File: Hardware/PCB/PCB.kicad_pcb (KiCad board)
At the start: 2 copper layers, 99.3 x 73.5 mm, 22 parts, among them J1 Conn_01x05_Pin, P1 USB_C_Plug, SW1 SW_HotSwap, U2 LP2985-3.3, U3 STM32F303RETx

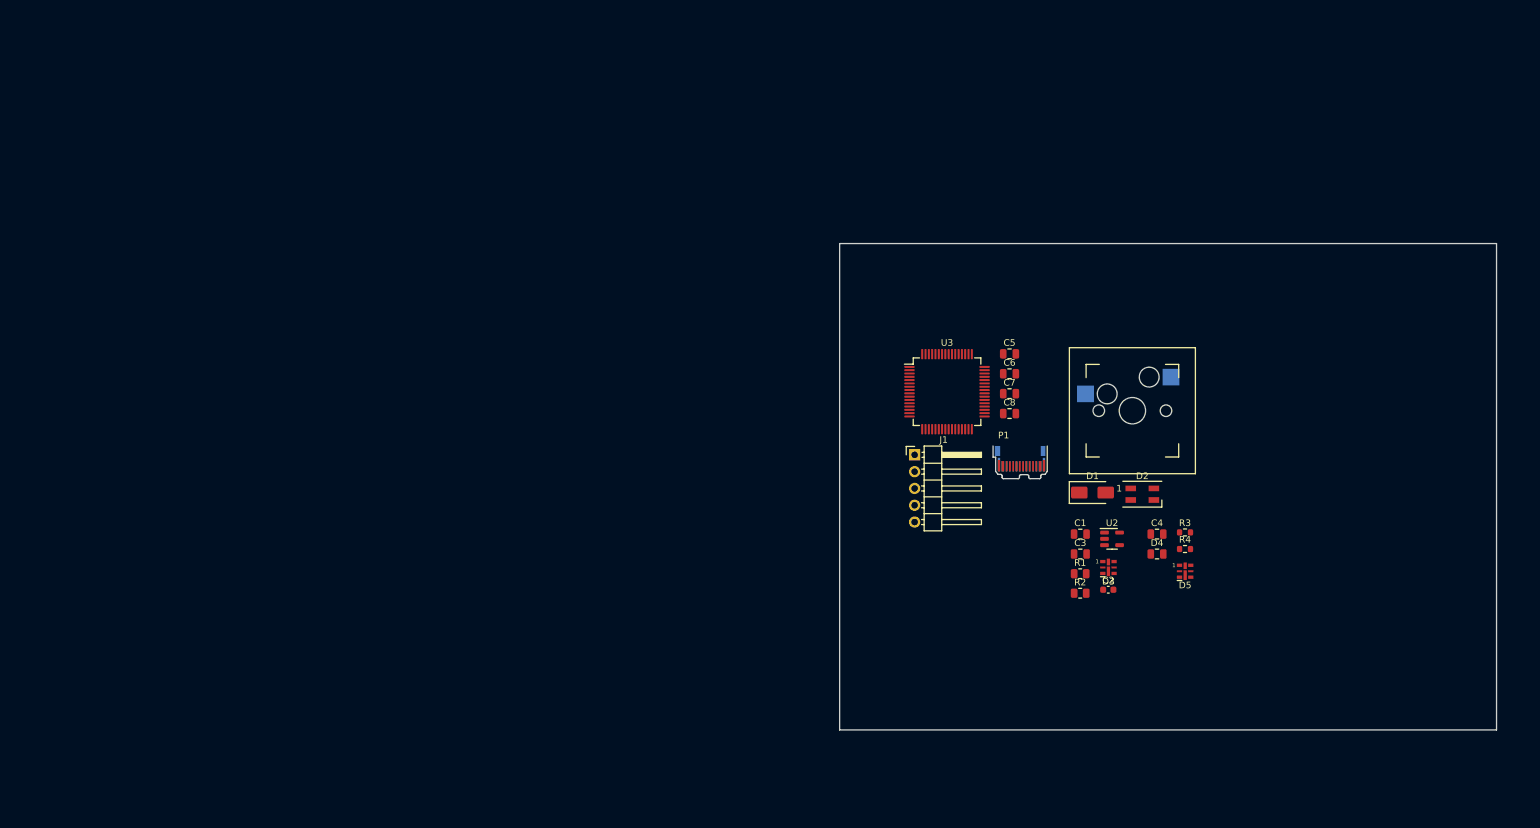
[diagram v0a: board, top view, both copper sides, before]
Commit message: Update of schematic and PCB
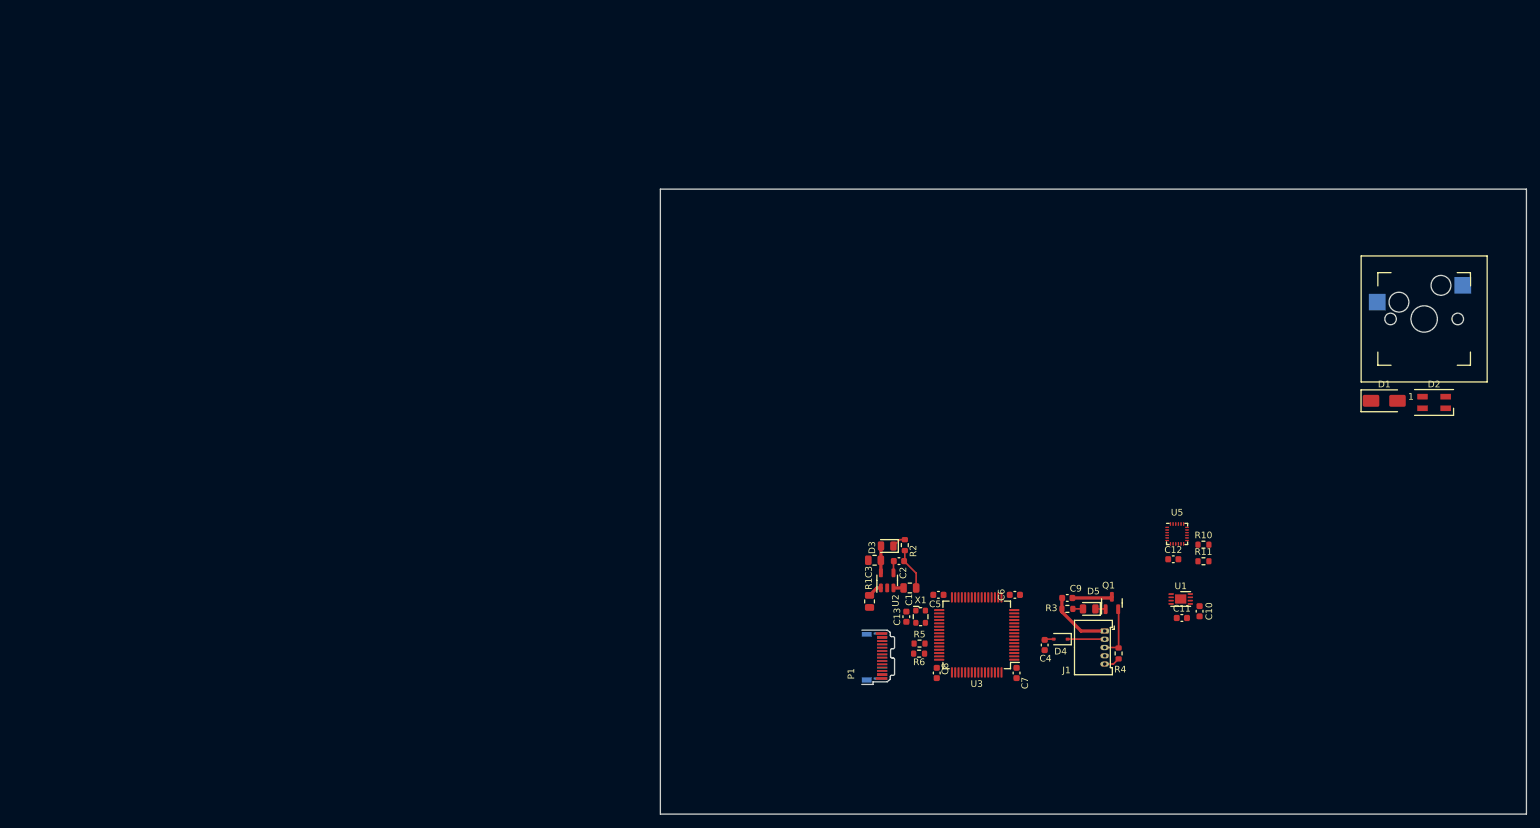
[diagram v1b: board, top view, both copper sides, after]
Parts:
- added C10: 100nF, Capacitor_SMD:C_0603_1608Metric, F.Cu at (199.0, 110.0)
- added C11: 100nF, Capacitor_SMD:C_0603_1608Metric, F.Cu at (196.3, 111.1)
- added C12: 100nF, Capacitor_SMD:C_0603_1608Metric, F.Cu at (195.0, 102.2)
- added C13: 100nF, Capacitor_SMD:C_0603_1608Metric, F.Cu at (154.7, 110.9)
- added C9: 100nF, Capacitor_SMD:C_0603_1608Metric, F.Cu at (179.0, 108.0)
- added Q1: NMOS, Package_TO_SOT_SMD:SOT-23, F.Cu at (185.7, 108.8)
- added R10: 4.7k, Resistor_SMD:R_0603_1608Metric, F.Cu at (199.6, 100.0)
- added R11: 4.7k, Resistor_SMD:R_0603_1608Metric, F.Cu at (199.6, 102.5)
- added R5: 0, Resistor_SMD:R_0603_1608Metric, F.Cu at (156.7, 114.9)
- added R6: 0, Resistor_SMD:R_0603_1608Metric, F.Cu at (156.6, 116.5)
- added U1: MCP98243, Package_DFN_QFN:DFN-8-1EP_3x2mm_P0.5mm_EP1.7x1.4mm, F.Cu at (196.1, 108.2)
- added U5: ICM-20948, Sensor_Motion:InvenSense_QFN-24_3x3mm_P0.4mm, F.Cu at (195.6, 98.4)
- added X1: ECS-2520MV-250-DN-TR, Oscillator:Oscillator_SMD_ECS_2520MV-xxx-xx-4Pin_2.5x2.0mm, F.Cu at (156.8, 110.9)
- C4, C5, C6, C7, C8: footprint Capacitor_SMD:C_0805_2012Metric -> Capacitor_SMD:C_0603_1608Metric
- D3, D5: footprint LED_SMD:LED-APA102-2020 -> LED_SMD:LED_0805_2012Metric
- D4: value 1N4818 -> BAS16HT1G; footprint Capacitor_SMD:C_0805_2012Metric -> Diode_SMD:D_SOD-323
- J1: value Conn_01x05_Pin -> 53048-0510; footprint Connector_PinHeader_2.54mm:PinHeader_1x05_P2.54mm_Horizontal -> Connector_Molex:Molex_PicoBlade_53048-0510_1x05_P1.25mm_Horizontal
- R2: footprint Resistor_SMD:R_0805_2012Metric -> Resistor_SMD:R_0603_1608Metric
- moved D1 46.2 mm to (226.9, 78.2)
- moved D2 46.2 mm to (234.4, 78.5)
- moved SW1 46.2 mm to (232.9, 65.9)
- moved C7 42.2 mm to (171.3, 119.4), turned to -90 degrees
- moved C8 40.7 mm to (159.3, 119.4), turned to 90 degrees
- moved J1 39.2 mm to (184.6, 113.0), turned to -90 degrees
- moved C5 38.0 mm to (159.5, 107.6), turned to 180 degrees
- moved P1 37.2 mm to (149.9, 116.8), turned to 90 degrees
- moved U3 37.0 mm to (165.3, 113.6), turned to 180 degrees
- moved U2 34.6 mm to (151.8, 105.4), turned to 90 degrees
- moved D3 33.6 mm to (151.8, 100.2), turned to 180 degrees
- moved C6 33.4 mm to (171.1, 107.6), turned to 180 degrees
- moved R1 32.1 mm to (149.1, 108.6), turned to 90 degrees
- moved C2 31.9 mm to (153.5, 102.5)
- moved C3 31.1 mm to (149.9, 102.3), turned to 180 degrees
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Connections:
- C4 pad 1: /Programming/NRST_OUT -> /MCU/NRST
- C5 pad 1: +3.3V -> /MCU/VCC_IN
- C6 pad 1: +3.3V -> /MCU/VCC_IN
- C7 pad 1: +3.3V -> /MCU/VCC_IN
- C8 pad 1: +3.3V -> /MCU/VCC_IN
- D4 pad 2: /Programming/NRST_OUT -> /MCU/NRST
- U3 pad 1: +3.3V -> /MCU/VCC_IN
- U3 pad 13: +3.3V -> /MCU/VCC_IN
- U3 pad 19: +3.3V -> /MCU/VCC_IN
- U3 pad 32: +3.3V -> /MCU/VCC_IN
- U3 pad 44: unconnected-(U3-PA11-Pad44) -> Net-(U3-PA11)
- U3 pad 45: unconnected-(U3-PA12-Pad45) -> Net-(U3-PA12)
- U3 pad 48: +3.3V -> /MCU/VCC_IN
- U3 pad 5: unconnected-(U3-PF0-Pad5) -> Net-(U3-PF0)
- U3 pad 64: +3.3V -> /MCU/VCC_IN
- U3 pad 7: unconnected-(U3-NRST-Pad7) -> /MCU/NRST
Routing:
- net GND: track 0.00 -> 14.9 mm
- net +5V: track 0.00 -> 9.77 mm
- net /Programming/SWD_IN: track 0.00 -> 8.02 mm
- net /Programming/NRST_IN: track 0.00 -> 5.61 mm
- net +3.3V: track 0.00 -> 4.08 mm
- net Net-(U2-ON/~{OFF}): track 0.00 -> 3.71 mm
- net Net-(D3-K): track 0.00 -> 2.12 mm
- net Net-(U2-BP): track 0.00 -> 1.81 mm
- net Net-(D5-K): track 0.00 -> 1.56 mm
- net Net-(D5-A): track 0.00 -> 1.54 mm
- net /MCU/NRST: track 0.00 -> 1.41 mm
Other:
- board size 99.3 x 73.5 mm -> 130.9 x 94.5 mm

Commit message: Update schematic
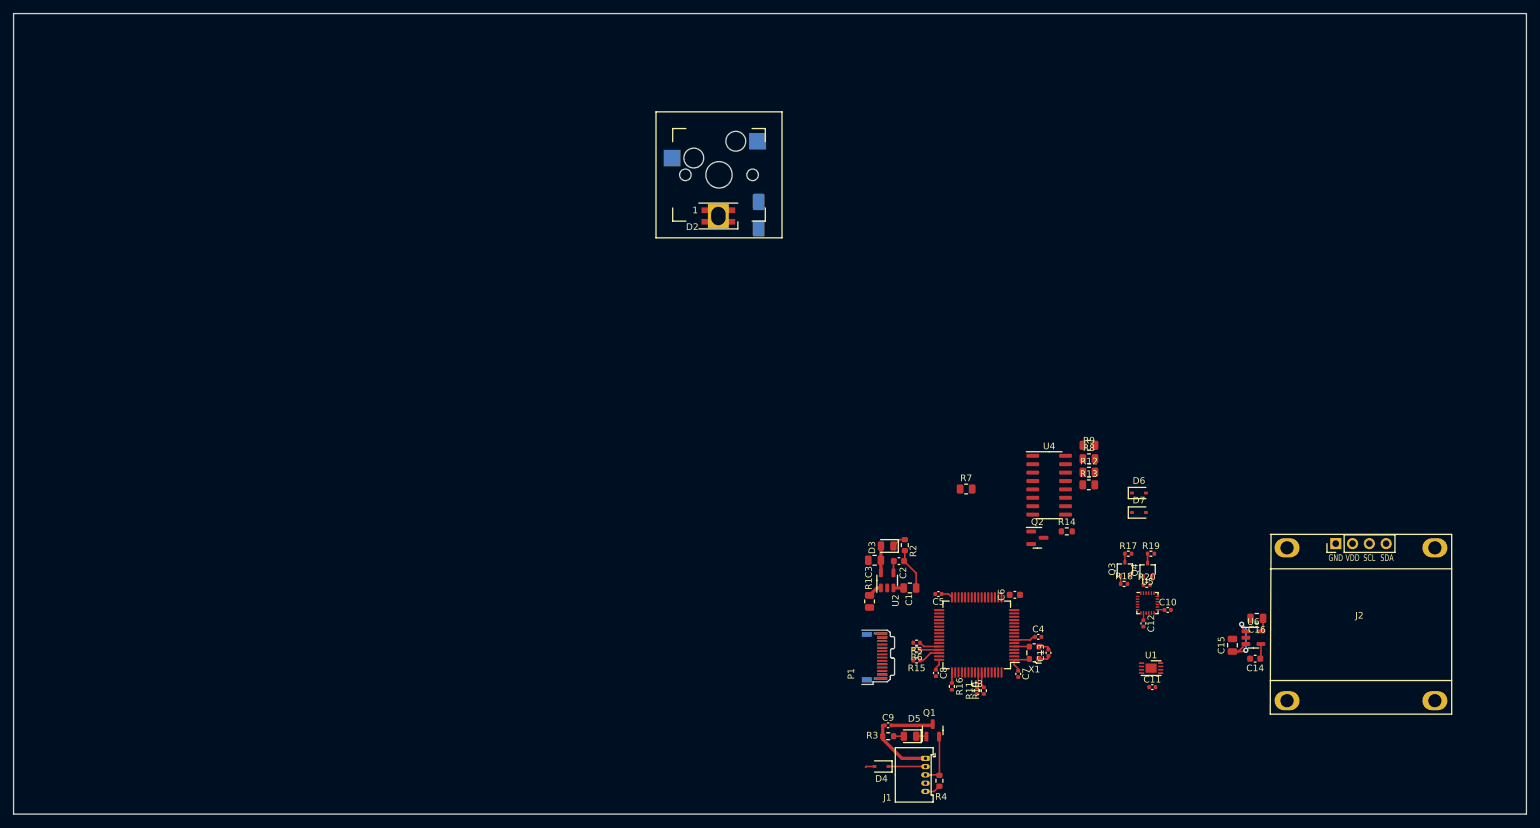
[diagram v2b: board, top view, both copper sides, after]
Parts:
- added C14: 10nF, Capacitor_SMD:C_0603_1608Metric, F.Cu at (207.4, 117.2)
- added C15: 2.2uF, Capacitor_SMD:C_0805_2012Metric, F.Cu at (204.0, 115.2)
- added C16: 4.7uF, Capacitor_SMD:C_0805_2012Metric, F.Cu at (207.6, 111.1)
- added D6: BAS16HT1G, Diode_SMD:D_SOD-323, F.Cu at (189.8, 92.2)
- added D7: Z3.3V, Diode_SMD:D_SOD-323, F.Cu at (189.8, 95.1)
- added J2: I2C_SSD1306, OLED:SSD1306_OLED_Display(128x64), F.Cu at (223.4, 99.8)
- added Q2: NMOS, Package_TO_SOT_SMD:SOT-23, F.Cu at (174.5, 98.9)
- added Q3: PJC138K_R1_00001, Package_TO_SOT_SMD:SOT-323_SC-70, F.Cu at (187.7, 103.6)
- added Q4: PJC138K_R1_00001, Package_TO_SOT_SMD:SOT-323_SC-70, F.Cu at (191.1, 103.8)
- added R12: 10k, Resistor_SMD:R_0805_2012Metric, F.Cu at (182.3, 89.0)
- added R13: 100k, Resistor_SMD:R_0805_2012Metric, F.Cu at (182.2, 90.9)
- added R14: 100k, Resistor_SMD:R_0603_1608Metric, F.Cu at (178.9, 98.0)
- added R15: 0, Resistor_SMD:R_0402_1005Metric, F.Cu at (156.2, 117.5)
- added R16: 0, Resistor_SMD:R_0402_1005Metric, F.Cu at (161.5, 121.4)
- added R17: 10k, Resistor_SMD:R_0402_1005Metric, F.Cu at (188.2, 101.3)
- added R18: 10k, Resistor_SMD:R_0402_1005Metric, F.Cu at (187.6, 105.9)
- added R19: 10k, Resistor_SMD:R_0402_1005Metric, F.Cu at (191.6, 101.3)
- added R20: 10k, Resistor_SMD:R_0402_1005Metric, F.Cu at (191.0, 106.0)
- added R7: 18, Resistor_SMD:R_0805_2012Metric, F.Cu at (163.7, 91.6)
- added R8: 1k, Resistor_SMD:R_0805_2012Metric, F.Cu at (182.3, 87.0)
- added R9: 100, Resistor_SMD:R_0805_2012Metric, F.Cu at (182.3, 85.0)
- added U4: MC1413BD, Package_SO:SOIC-16_3.9x9.9mm_P1.27mm, F.Cu at (176.3, 91.0)
- added U6: TC1015-1.8VCT713, Package_TO_SOT_SMD:SOT-23-5, F.Cu at (207.1, 114.0)
- C10, C11, C12, C13, C4, C5, C7, C8, C9: footprint Capacitor_SMD:C_0603_1608Metric -> Capacitor_SMD:C_0402_1005Metric
- D1: moved to B.Cu
- R10, R11, R5, R6: footprint Resistor_SMD:R_0603_1608Metric -> Resistor_SMD:R_0402_1005Metric
- moved D2 111.8 mm to (126.2, 50.3)
- moved SW1 108.8 mm to (126.3, 44.1)
- moved D1 98.7 mm to (132.3, 50.2), turned to -90 degrees
- moved R10 39.9 mm to (166.4, 122.0), turned to 90 degrees
- moved R11 39.4 mm to (165.4, 122.0), turned to 90 degrees
- moved J1 33.2 mm to (157.6, 132.3)
- moved Q1 33.2 mm to (158.6, 128.1)
- moved C9 33.2 mm to (151.9, 127.3)
- moved D4 33.2 mm to (150.9, 133.5)
- moved D5 33.2 mm to (155.2, 128.9)
- moved R3 33.2 mm to (151.9, 128.9)
- moved R4 33.2 mm to (159.7, 135.7)
- moved C13 22.2 mm to (176.1, 116.3), turned to 90 degrees
- moved X1 18.0 mm to (174.0, 116.3), turned to 180 degrees
- moved U1 11.4 mm to (191.7, 118.6)
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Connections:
- net +5V renamed /Programming/+5V_IN
- net /Programming/SWD_IN renamed /MCU/SWD
- C10 pad 1: +3.3V -> /IMU/+3.3V
- C11 pad 1: /MCU/VCC_IN -> /Multimeter/VCC_IN
- C11 pad 2: /Temperature/GND_IMU -> /Temperature/GND
- C12 pad 1: +3.3V -> /IMU/+3.3V
- C13 pad 1: /MCU/VCC_IN -> /MCU/+3.3V
- C13 pad 2: GND -> /MCU/GND
- C3 pad 1: +3.3V -> /Multimeter/VCC_IN
- C5 pad 1: /MCU/VCC_IN -> /MCU/+3.3V
- C5 pad 2: GND -> /MCU/GND
- C6 pad 1: /MCU/VCC_IN -> /MCU/+3.3V
- C6 pad 2: GND -> /MCU/GND
- C7 pad 1: /MCU/VCC_IN -> /MCU/+3.3V
- C7 pad 2: GND -> /MCU/GND
- C8 pad 1: /MCU/VCC_IN -> /MCU/+3.3V
- C8 pad 2: GND -> /MCU/GND
- D2 pad 2: GND -> /Key_1U/GND
- D3 pad 2: +3.3V -> /Multimeter/VCC_IN
- J1 pad 4: /Programming/SWC_IN -> /MCU/SWC
- R10 pad 2: /MCU/SCL_MCU -> /IMU/SCL
- R11 pad 2: /MCU/SDA_MCU -> /IMU/SDA
- U1 pad 1: /Temperature/TMP_SDA -> /IMU/SDA
- U1 pad 2: /Temperature/TMP_SCL -> /IMU/SCL
- U1 pad 4: /Temperature/GND_TMP -> /Temperature/GND
- U1 pad 8: /MCU/VCC_IN -> /Multimeter/VCC_IN
- U1 pad 9: /Temperature/GND_TMP -> /Temperature/GND
- U2 pad 5: +3.3V -> /Multimeter/VCC_IN
- U3 pad 1: /MCU/VCC_IN -> /MCU/+3.3V
- U3 pad 12: GND -> /MCU/GND
- U3 pad 13: /MCU/VCC_IN -> /MCU/+3.3V
- U3 pad 18: GND -> /MCU/GND
- U3 pad 19: /MCU/VCC_IN -> /MCU/+3.3V
- U3 pad 31: GND -> /MCU/GND
- U3 pad 32: /MCU/VCC_IN -> /MCU/+3.3V
- U3 pad 46: unconnected-(U3-PA13-Pad46) -> Net-(U3-PA13)
- U3 pad 47: GND -> /MCU/GND
- U3 pad 48: /MCU/VCC_IN -> /MCU/+3.3V
- U3 pad 49: unconnected-(U3-PA14-Pad49) -> Net-(U3-PA14)
- U3 pad 57: unconnected-(U3-PB5-Pad57) -> /IMU/SDA
- U3 pad 58: unconnected-(U3-PB6-Pad58) -> /IMU/SCL
- U3 pad 63: GND -> /MCU/GND
- U3 pad 64: /MCU/VCC_IN -> /MCU/+3.3V
- U5 pad 12: unconnected-(U5-INT1-Pad12) -> GND
- U5 pad 13: +3.3V -> /IMU/+3.3V
- U5 pad 23: /IMU/IMU_SCL -> /IMU/I2C_LevelShifter/SCL_LL
- U5 pad 24: /IMU/IMU_SDA -> /IMU/I2C_LevelShifter/SDA_LL
- U5 pad 8: +3.3V -> /IMU/+3.3V
- X1 pad 1: /MCU/VCC_IN -> /MCU/+3.3V
- X1 pad 2: GND -> /MCU/GND
- X1 pad 4: /MCU/VCC_IN -> /MCU/+3.3V
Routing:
- net Net-(U2-ON/~{OFF}): track 3.71 -> 13.9 mm, vias 0 -> 2
- net /MCU/+3.3V: track 0.00 -> 8.36 mm
- net /Multimeter/VCC_IN: track 0.00 -> 4.08 mm
- net +3.3V: track 4.08 -> 0.00 mm
- net /IMU/SCL: track 0.00 -> 3.79 mm
- net /IMU/SDA: track 0.00 -> 3.61 mm
- net Net-(U3-PA13): track 0.00 -> 3.36 mm
- net Net-(U3-PA11): track 0.00 -> 3.14 mm
- net /MCU/NRST: track 1.41 -> 4.46 mm
- net Net-(U3-PA12): track 0.00 -> 2.93 mm
- net Net-(U3-PF0): track 0.00 -> 2.30 mm
- net Net-(U6-Bypass): track 0.00 -> 2.26 mm
- net /IMU/+3.3V: track 0.00 -> 2.20 mm
- net /Supply/+1.8V: track 0.00 -> 2.10 mm
- net Net-(U3-PA14): track 0.00 -> 1.61 mm
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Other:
- board size 130.9 x 94.5 mm -> 228.7 x 121 mm
